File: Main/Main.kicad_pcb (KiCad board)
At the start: 2 copper layers, 147.3 x 70.6 mm, 60 parts, among them J1 Conn_02x03_Odd_Even, J2 Conn_01x06, J3 Conn_01x03, J4 Conn_01x02, J5 Conn_01x12, J6 Conn_01x06, Q1 BCP56, SW1 SW_Push, SW2 SW_Push, SW3 SW_Push, U1 LM358, U2 ATmega324PA-AU, U3 TLV1117-33, U4 DEM128064F, X1 20MHz

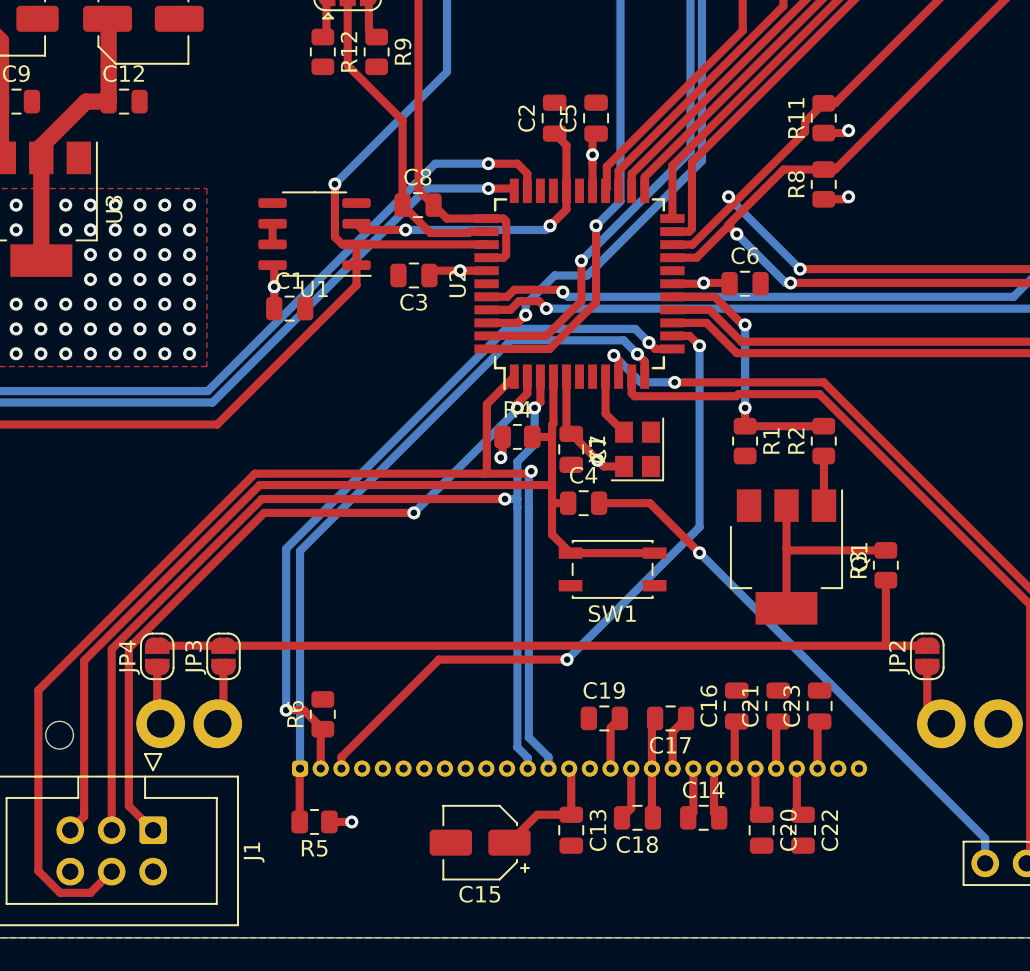
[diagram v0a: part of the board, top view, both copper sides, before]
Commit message: Triac board updated
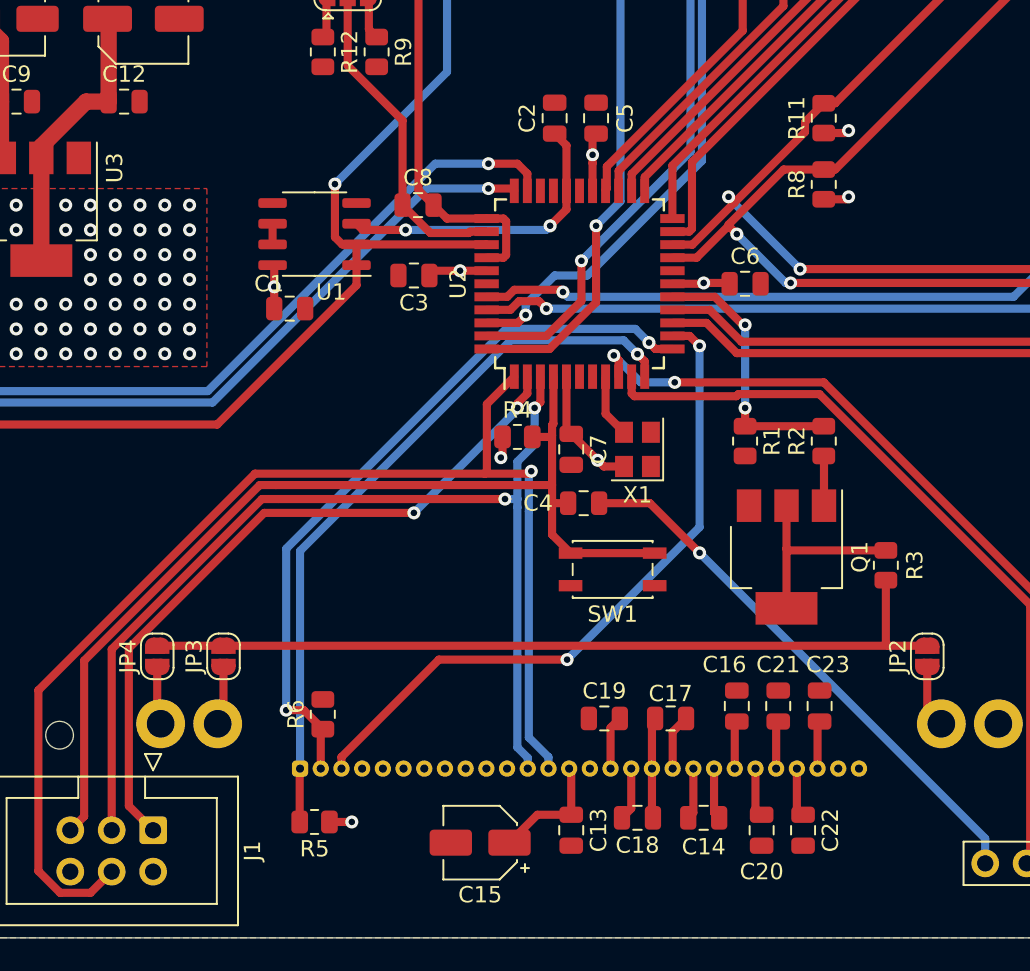
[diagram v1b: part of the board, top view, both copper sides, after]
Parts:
- H1, H2, H3, H4: footprint MountingHole:MountingHole_3.2mm_M3 -> Thermostat:MountingHole_3.2mm_M3
